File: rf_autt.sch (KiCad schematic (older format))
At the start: 10 parts

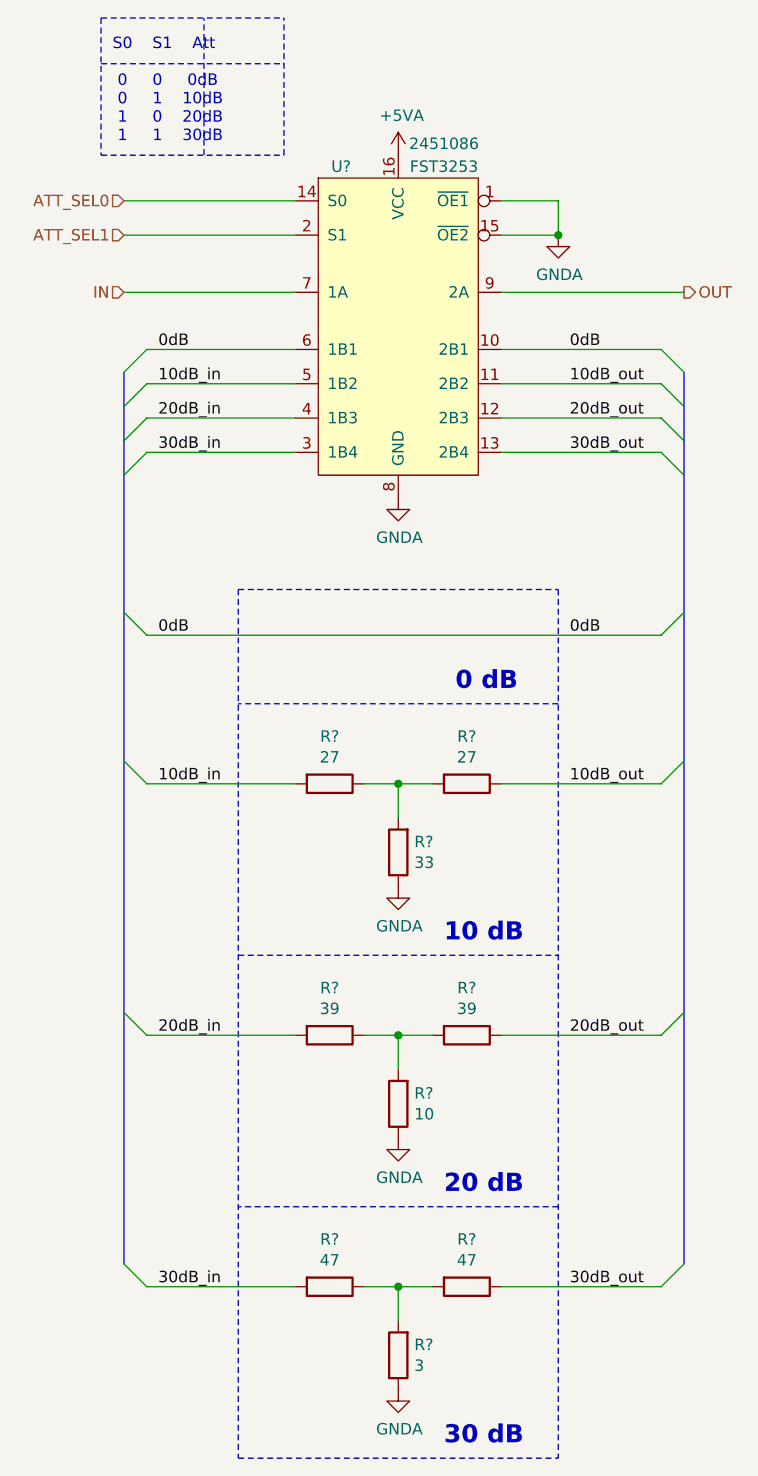
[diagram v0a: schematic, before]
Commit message: PCB is Done... Needs DRC check
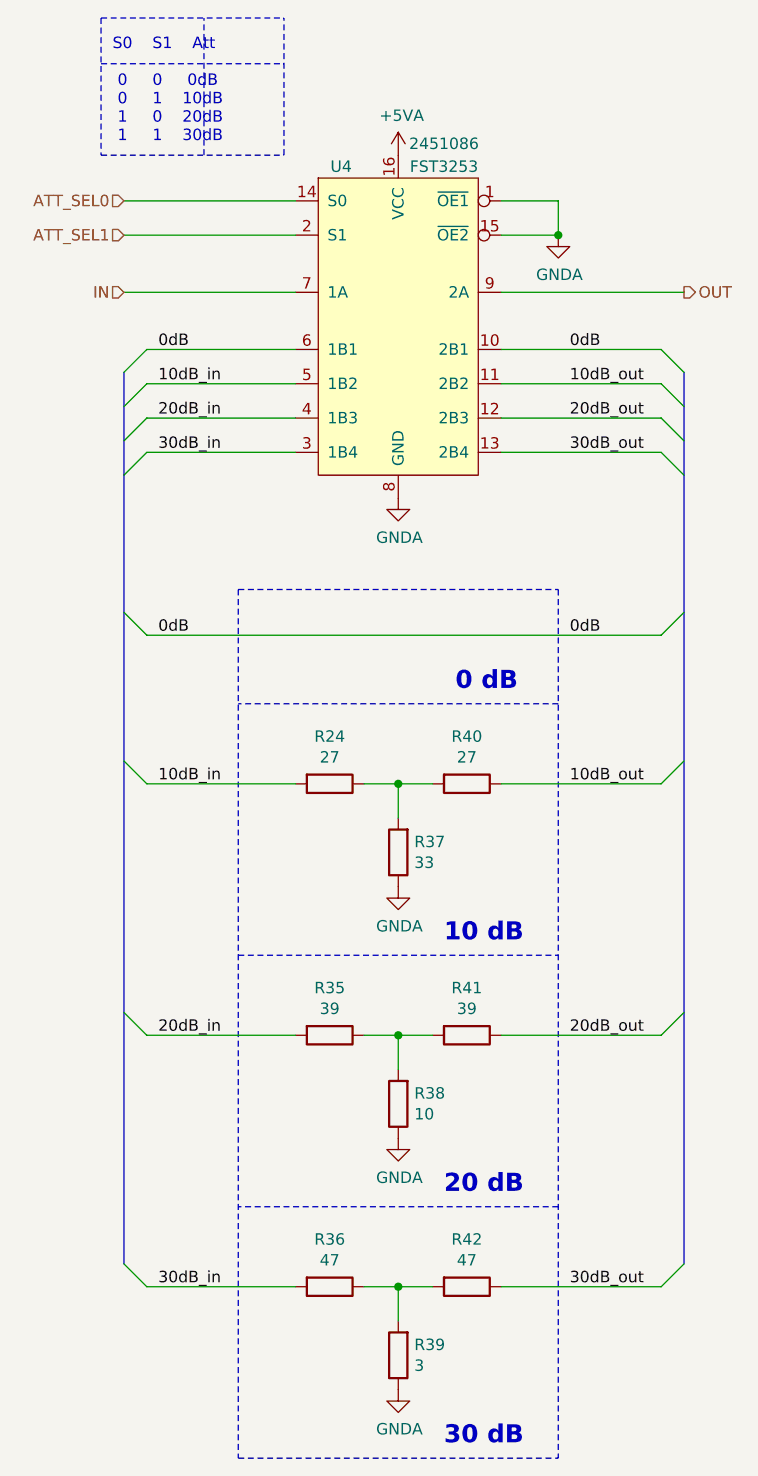
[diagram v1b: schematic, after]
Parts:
- gave numbers to parts that had none: 10
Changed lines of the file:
@@
 $Descr A4 11693 8268
 encoding utf-8
-Sheet 7 14
+Sheet 7 7
 Title "HF-SDR RF-Attenuator"
 Date "2020 december"
@@
 OUT
 $Comp
-L sdr:FST3253 U?
+L sdr:FST3253 U4
 U 1 1 5FE50A6B
 P 5600 1900
-F 0 "U?" H 5350 2550 50  0000 C CNN
+F 0 "U4" H 5350 2550 50  0000 C CNN
 F 1 "FST3253" H 5800 2550 50  0000 C CNN
 F 2 "Package_SO:TSSOP-16_4.4x5mm_P0.65mm" H 5600 1900 50  0001 C CNN
@@
 ATT_SEL1
 $Comp
-L power:GNDA #PWR?
+L power:GNDA #PWR031
 U 1 1 5FE53082
 P 5600 4400
-F 0 "#PWR?" H 5600 4150 50  0001 C CNN
+F 0 "#PWR031" H 5600 4150 50  0001 C CNN
 F 1 "GNDA" H 5605 4227 50  0000 C CNN
 F 2 "" H 5600 4400 50  0001 C CNN
@@
 $EndComp
 $Comp
-L Device:R R?
+L Device:R R37
 U 1 1 5FE56E4E
 P 5600 4250
-F 0 "R?" H 5530 4204 50  0000 R CNN
+F 0 "R37" H 5530 4204 50  0000 R CNN
 F 1 "33" H 5530 4295 50  0000 R CNN
 F 2 "Resistor_SMD:R_0805_2012Metric_Pad1.20x1.40mm_HandSolder" V 5530 4250 50  0001 C CNN
@@
 $EndComp
 $Comp
-L Device:R R?
+L Device:R R24
 U 1 1 5FE5744A
 P 5300 3950
-F 0 "R?" V 5093 3950 50  0000 C CNN
+F 0 "R24" V 5093 3950 50  0000 C CNN
 F 1 "27" V 5184 3950 50  0000 C CNN
 F 2 "Resistor_SMD:R_0805_2012Metric_Pad1.20x1.40mm_HandSolder" V 5230 3950 50  0001 C CNN
@@
 $EndComp
 $Comp
-L Device:R R?
+L Device:R R40
 U 1 1 5FE57E99
 P 5900 3950
-F 0 "R?" V 5693 3950 50  0000 C CNN
+F 0 "R40" V 5693 3950 50  0000 C CNN
 F 1 "27" V 5784 3950 50  0000 C CNN
 F 2 "Resistor_SMD:R_0805_2012Metric_Pad1.20x1.40mm_HandSolder" V 5830 3950 50  0001 C CNN
@@
 	5600 3950 5750 3950
 $Comp
-L power:GNDA #PWR?
+L power:GNDA #PWR033
 U 1 1 5FE5C53B
 P 5600 6600
-F 0 "#PWR?" H 5600 6350 50  0001 C CNN
+F 0 "#PWR033" H 5600 6350 50  0001 C CNN
 F 1 "GNDA" H 5605 6427 50  0000 C CNN
 F 2 "" H 5600 6600 50  0001 C CNN
@@
 $EndComp
 $Comp
-L Device:R R?
+L Device:R R39
 U 1 1 5FE5C541
 P 5600 6450
-F 0 "R?" H 5530 6404 50  0000 R CNN
+F 0 "R39" H 5530 6404 50  0000 R CNN
 F 1 "3" H 5530 6495 50  0000 R CNN
 F 2 "Resistor_SMD:R_0805_2012Metric_Pad1.20x1.40mm_HandSolder" V 5530 6450 50  0001 C CNN
@@
 $EndComp
 $Comp
-L Device:R R?
+L Device:R R36
 U 1 1 5FE5C547
 P 5300 6150
-F 0 "R?" V 5093 6150 50  0000 C CNN
+F 0 "R36" V 5093 6150 50  0000 C CNN
 F 1 "47" V 5184 6150 50  0000 C CNN
 F 2 "Resistor_SMD:R_0805_2012Metric_Pad1.20x1.40mm_HandSolder" V 5230 6150 50  0001 C CNN
@@
 $EndComp
 $Comp
-L Device:R R?
+L Device:R R42
 U 1 1 5FE5C54D
 P 5900 6150
-F 0 "R?" V 5693 6150 50  0000 C CNN
+F 0 "R42" V 5693 6150 50  0000 C CNN
 F 1 "47" V 5784 6150 50  0000 C CNN
 F 2 "Resistor_SMD:R_0805_2012Metric_Pad1.20x1.40mm_HandSolder" V 5830 6150 50  0001 C CNN
@@
 	5600 6150 5750 6150
 $Comp
-L power:GNDA #PWR?
+L power:GNDA #PWR032
 U 1 1 5FE5CA2D
 P 5600 5500
-F 0 "#PWR?" H 5600 5250 50  0001 C CNN
+F 0 "#PWR032" H 5600 5250 50  0001 C CNN
 F 1 "GNDA" H 5605 5327 50  0000 C CNN
 F 2 "" H 5600 5500 50  0001 C CNN
@@
 $EndComp
 $Comp
-L Device:R R?
+L Device:R R38
 U 1 1 5FE5CA33
 P 5600 5350
-F 0 "R?" H 5530 5304 50  0000 R CNN
+F 0 "R38" H 5530 5304 50  0000 R CNN
 F 1 "10" H 5530 5395 50  0000 R CNN
 F 2 "Resistor_SMD:R_0805_2012Metric_Pad1.20x1.40mm_HandSolder" V 5530 5350 50  0001 C CNN
@@
 $EndComp
 $Comp
-L Device:R R?
+L Device:R R35
 U 1 1 5FE5CA39
 P 5300 5050
-F 0 "R?" V 5093 5050 50  0000 C CNN
+F 0 "R35" V 5093 5050 50  0000 C CNN
 F 1 "39" V 5184 5050 50  0000 C CNN
 F 2 "Resistor_SMD:R_0805_2012Metric_Pad1.20x1.40mm_HandSolder" V 5230 5050 50  0001 C CNN
@@
 $EndComp
 $Comp
-L Device:R R?
+L Device:R R41
 U 1 1 5FE5CA3F
 P 5900 5050
-F 0 "R?" V 5693 5050 50  0000 C CNN
+F 0 "R41" V 5693 5050 50  0000 C CNN
 F 1 "39" V 5784 5050 50  0000 C CNN
 F 2 "Resistor_SMD:R_0805_2012Metric_Pad1.20x1.40mm_HandSolder" V 5830 5050 50  0001 C CNN
@@
 	4300 800  5100 800
 $Comp
-L power:GNDA #PWR?
+L power:GNDA #PWR030
 U 1 1 5FF9D7B5
 P 5600 2700
-F 0 "#PWR?" H 5600 2450 50  0001 C CNN
+F 0 "#PWR030" H 5600 2450 50  0001 C CNN
 F 1 "GNDA" H 5605 2527 50  0000 C CNN
 F 2 "" H 5600 2700 50  0001 C CNN
@@
 $EndComp
 $Comp
-L power:GNDA #PWR?
+L power:GNDA #PWR034
 U 1 1 5FF9DC72
 P 6300 1550
-F 0 "#PWR?" H 6300 1300 50  0001 C CNN
+F 0 "#PWR034" H 6300 1300 50  0001 C CNN
 F 1 "GNDA" H 6305 1377 50  0000 C CNN
 F 2 "" H 6300 1550 50  0001 C CNN
@@
 Connection ~ 6300 1550
 $Comp
-L power:+5VA #PWR?
+L power:+5VA #PWR029
 U 1 1 5FF9E701
 P 5600 1200
-F 0 "#PWR?" H 5600 1050 50  0001 C CNN
+F 0 "#PWR029" H 5600 1050 50  0001 C CNN
 F 1 "+5VA" H 5615 1373 50  0000 C CNN
 F 2 "" H 5600 1200 50  0001 C CNN
